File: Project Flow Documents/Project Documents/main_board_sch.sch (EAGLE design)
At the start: 61 parts, among them IC3 LM2936MP-3.3, Q1 8meg, Q2 2N3904, Q4 2N3704, X1 SDBMF

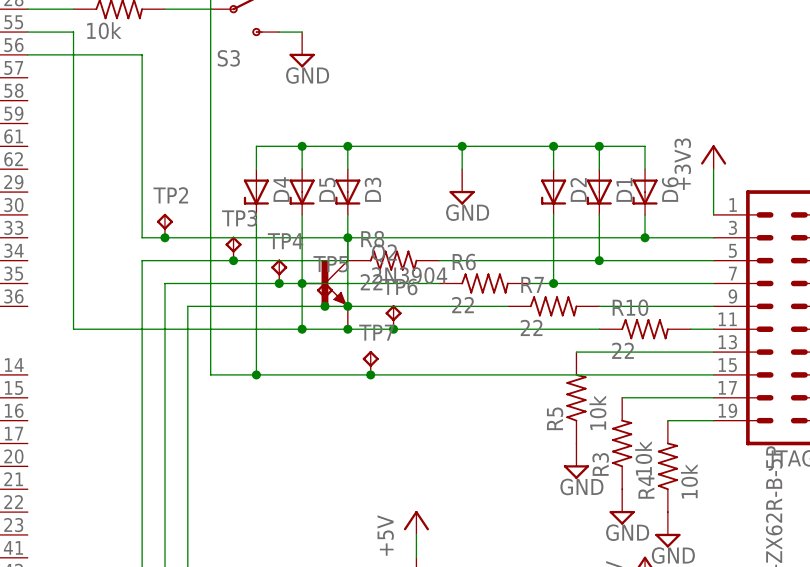
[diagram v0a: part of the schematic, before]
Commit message: Small Corrections
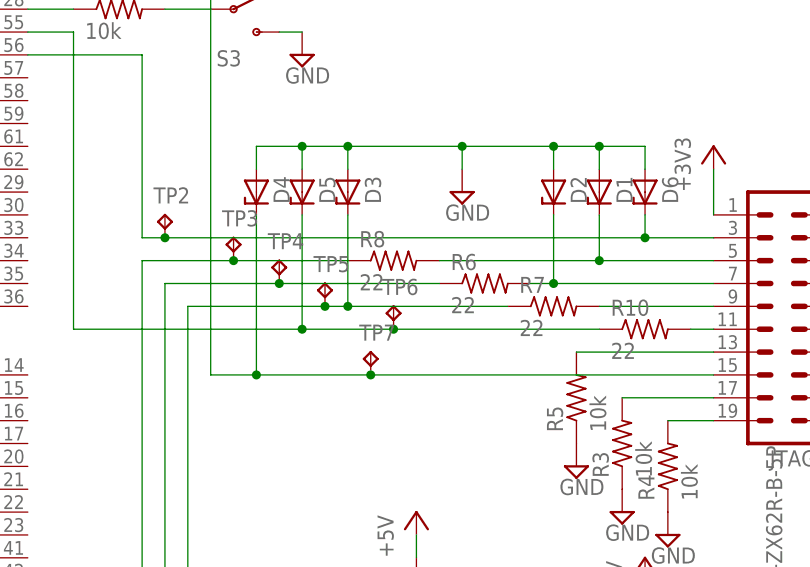
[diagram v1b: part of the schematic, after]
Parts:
- removed Q2: 2N3904, transistor-small-signal:2N3904
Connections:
- net N$10: no longer Q2.B
- net N$12: no longer Q2.E
- net N$8: no longer Q2.C
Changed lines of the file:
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@@
 <part name="SUPPLY36" library="supply2" deviceset="GND" device=""/>
 <part name="P+1" library="supply1" deviceset="+5V" device=""/>
-<part name="Q2" library="transistor-small-signal" deviceset="2N3904" device=""/>
 <part name="Q4" library="transistor-small-signal" deviceset="2N3704" device=""/>
 <part name="R16" library="rcl" deviceset="R-US_" device="R0805" value="10k"/>
@@
 <instance part="SUPPLY36" gate="GND" x="203.2" y="38.1"/>
 <instance part="P+1" gate="1" x="203.2" y="71.12"/>
-<instance part="Q2" gate="1" x="167.64" y="101.6"/>
 <instance part="Q4" gate="1" x="185.42" y="50.8"/>
 <instance part="R16" gate="G$1" x="177.8" y="43.18" rot="R90"/>
@@
 <wire x1="147.32" y1="106.68" x2="149.86" y2="106.68" width="0.1524" layer="91"/>
 <pinref part="D6" gate="G$1" pin="C"/>
-<wire x1="149.86" y1="106.68" x2="170.18" y2="106.68" width="0.1524" layer="91"/>
-<wire x1="170.18" y1="106.68" x2="203.2" y2="106.68" width="0.1524" layer="91"/>
+<wire x1="149.86" y1="106.68" x2="203.2" y2="106.68" width="0.1524" layer="91"/>
 <wire x1="203.2" y1="106.68" x2="210.82" y2="106.68" width="0.1524" layer="91"/>
 <wire x1="203.2" y1="109.22" x2="203.2" y2="106.68" width="0.1524" layer="91"/>
@@
 <pinref part="TP2" gate="G$1" pin="TP"/>
 <junction x="149.86" y="106.68"/>
-<pinref part="Q2" gate="1" pin="C"/>
-<junction x="170.18" y="106.68"/>
 </segment>
 </net>
@@
 <pinref part="R6" gate="G$1" pin="1"/>
 <pinref part="TP4" gate="G$1" pin="TP"/>
-<wire x1="162.56" y1="101.6" x2="165.1" y2="101.6" width="0.1524" layer="91"/>
 <junction x="162.56" y="101.6"/>
-<pinref part="Q2" gate="1" pin="B"/>
-<wire x1="165.1" y1="101.6" x2="180.34" y2="101.6" width="0.1524" layer="91"/>
-<junction x="165.1" y="101.6"/>
+<wire x1="162.56" y1="101.6" x2="180.34" y2="101.6" width="0.1524" layer="91"/>
 </segment>
 </net>
@@
 <pinref part="R10" gate="G$1" pin="1"/>
 <wire x1="198.12" y1="96.52" x2="175.26" y2="96.52" width="0.1524" layer="91"/>
-<wire x1="175.26" y1="96.52" x2="170.18" y2="96.52" width="0.1524" layer="91"/>
-<wire x1="170.18" y1="96.52" x2="165.1" y2="96.52" width="0.1524" layer="91"/>
+<wire x1="175.26" y1="96.52" x2="165.1" y2="96.52" width="0.1524" layer="91"/>
 <wire x1="165.1" y1="96.52" x2="139.7" y2="96.52" width="0.1524" layer="91"/>
 <wire x1="165.1" y1="109.22" x2="165.1" y2="96.52" width="0.1524" layer="91"/>
@@
 <pinref part="TP6" gate="G$1" pin="TP"/>
 <junction x="175.26" y="96.52"/>
-<pinref part="Q2" gate="1" pin="E"/>
-<junction x="170.18" y="96.52"/>
-</segment>
-</net>
+</segment>
+</net>
